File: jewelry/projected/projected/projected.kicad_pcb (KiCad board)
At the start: 2 copper layers, 28 x 28 mm, 38 parts, among them Q1 BC847, U1 STM32L432KBU6, U2 MCP73812T-420I-OT, U3 PCA9306DCUR, U4 MCP1640BCH, U5 TPS7A0533, U6 LIS2DE12

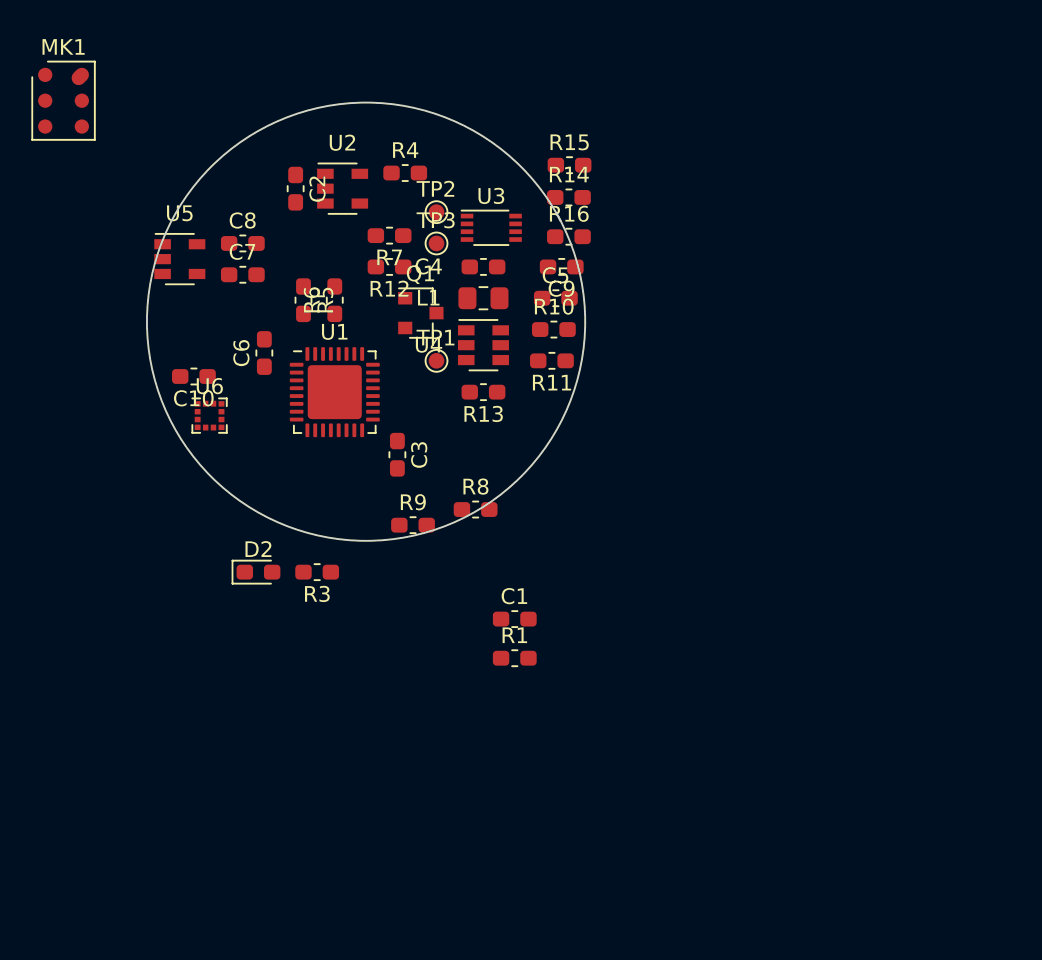
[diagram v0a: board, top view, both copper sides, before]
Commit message: projected: Layout nearly done
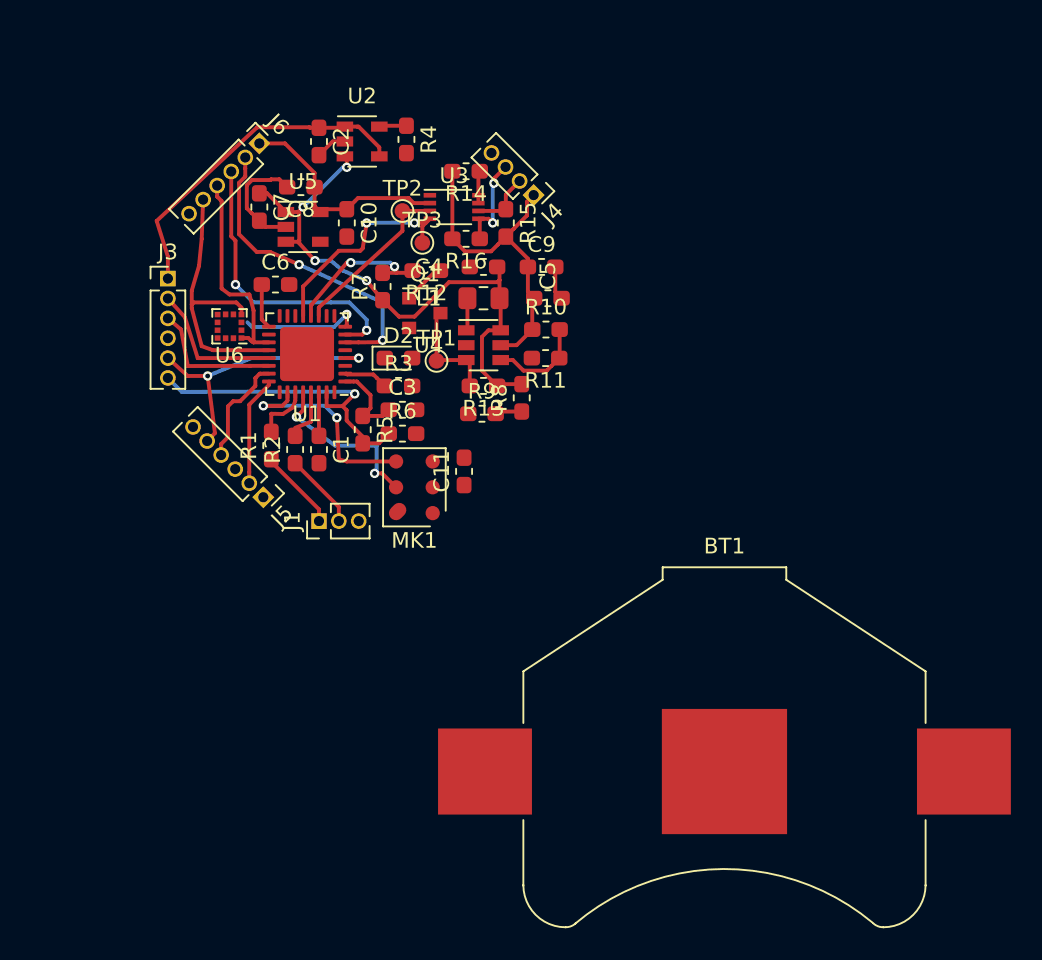
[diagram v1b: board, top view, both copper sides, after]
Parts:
- added BT1: LIR2450, Battery:BatteryHolder_Keystone_3008_1x2450, F.Cu at (72.9, 78.7)
- added C11: 1uF, Capacitor_SMD:C_0603_1608Metric_Pad1.05x0.95mm_HandSolder, F.Cu at (56.3, 59.6)
- added J1: TOUCH, Connector_PinHeader_1.27mm:PinHeader_1x03_P1.27mm_Vertical, F.Cu at (47.0, 62.7)
- added J3: DOCK, Connector_PinHeader_1.27mm:PinHeader_1x06_P1.27mm_Vertical, F.Cu at (37.3, 47.2)
- added J4: Leds, Connector_PinHeader_1.27mm:PinHeader_1x04_P1.27mm_Vertical, F.Cu at (60.7, 41.9)
- added J5: SWD, Connector_PinHeader_1.27mm:PinHeader_1x06_P1.27mm_Vertical, F.Cu at (43.4, 61.2)
- added J6: EXT, Connector_PinHeader_1.27mm:PinHeader_1x06_P1.27mm_Vertical, F.Cu at (43.2, 38.6)
- added R2: 1k, Resistor_SMD:R_0603_1608Metric_Pad1.05x0.95mm_HandSolder, F.Cu at (45.5, 58.2)
- R1: value R -> 1k
- moved MK1 33.4 mm to (53.1, 60.6), turned to 180 degrees
- moved R1 20.7 mm to (43.9, 57.9), turned to 90 degrees
- moved C1 16.5 mm to (47.0, 58.2), turned to 270 degrees
- moved D2 16.3 mm to (52.1, 52.3)
- moved C10 13.8 mm to (48.8, 43.7), turned to 270 degrees
- moved R3 13.0 mm to (52.1, 54.1), turned to 0 degrees
- moved R6 9.56 mm to (52.3, 57.1), turned to 0 degrees
- moved R5 9.10 mm to (49.8, 56.9)
- moved R9 8.37 mm to (57.4, 55.9)
- moved U5 8.14 mm to (46.0, 43.9)
- moved R8 7.72 mm to (59.9, 54.9), turned to 90 degrees
- moved R14 6.78 mm to (56.4, 40.4), turned to 180 degrees
- moved R16 6.57 mm to (56.4, 44.7), turned to 180 degrees
- moved U6 5.85 mm to (41.3, 50.3), turned to 180 degrees
- moved R15 5.49 mm to (58.9, 43.7), turned to 270 degrees
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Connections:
- C1 pad 1: Net-(C1-Pad1) -> /TOUCH_CS
- C1 pad 2: Net-(C1-Pad2) -> GND
- R1 pad 2: Net-(R1-Pad2) -> /TOUCH_1
- U1 pad 12: Net-(U1-Pad12) -> /LED_ENABLE
- U1 pad 18: /LED_ENABLE -> Net-(U1-Pad18)
- U1 pad 25: /TOUCH_2 -> Net-(U1-Pad25)
- U1 pad 27: Net-(U1-Pad27) -> /TOUCH_1
- U1 pad 29: Net-(U1-Pad29) -> /TOUCH_2
- U1 pad 30: /TOUCH_1 -> /TOUCH_CS
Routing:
- net +BATT: track 0.00 -> 37.4 mm, vias 0 -> 4
- net VCC: track 0.00 -> 22.7 mm
- net VBUS: track 0.00 -> 21.5 mm
- net +5V: track 0.00 -> 21.0 mm
- net /ANALOG+: track 0.00 -> 20.2 mm, vias 0 -> 2
- net /BOOT: track 0.00 -> 20.2 mm, vias 0 -> 1
- net /ANALOG-: track 0.00 -> 18.8 mm, vias 0 -> 2
- net /RESET: track 0.00 -> 18.1 mm, vias 0 -> 2
- net /I2C_SDA: track 0.00 -> 17.7 mm
- net /LED_DATA: track 0.00 -> 14.2 mm, vias 0 -> 2
- net /SAI_SCK: track 0.00 -> 13.6 mm, vias 0 -> 2
- net /I2C_SCL: track 0.00 -> 13.5 mm
- net /SAI_SD: track 0.00 -> 11.0 mm, vias 0 -> 2
- net /LED_CLK: track 0.00 -> 10.8 mm
- net /LED_ENABLE: track 0.00 -> 9.81 mm, vias 0 -> 2
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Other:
- board outline removed
- net class Default: via_dia 0.8 -> 0.6; via_drill 0.4 -> 0.3

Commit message: projected: Intial layout done
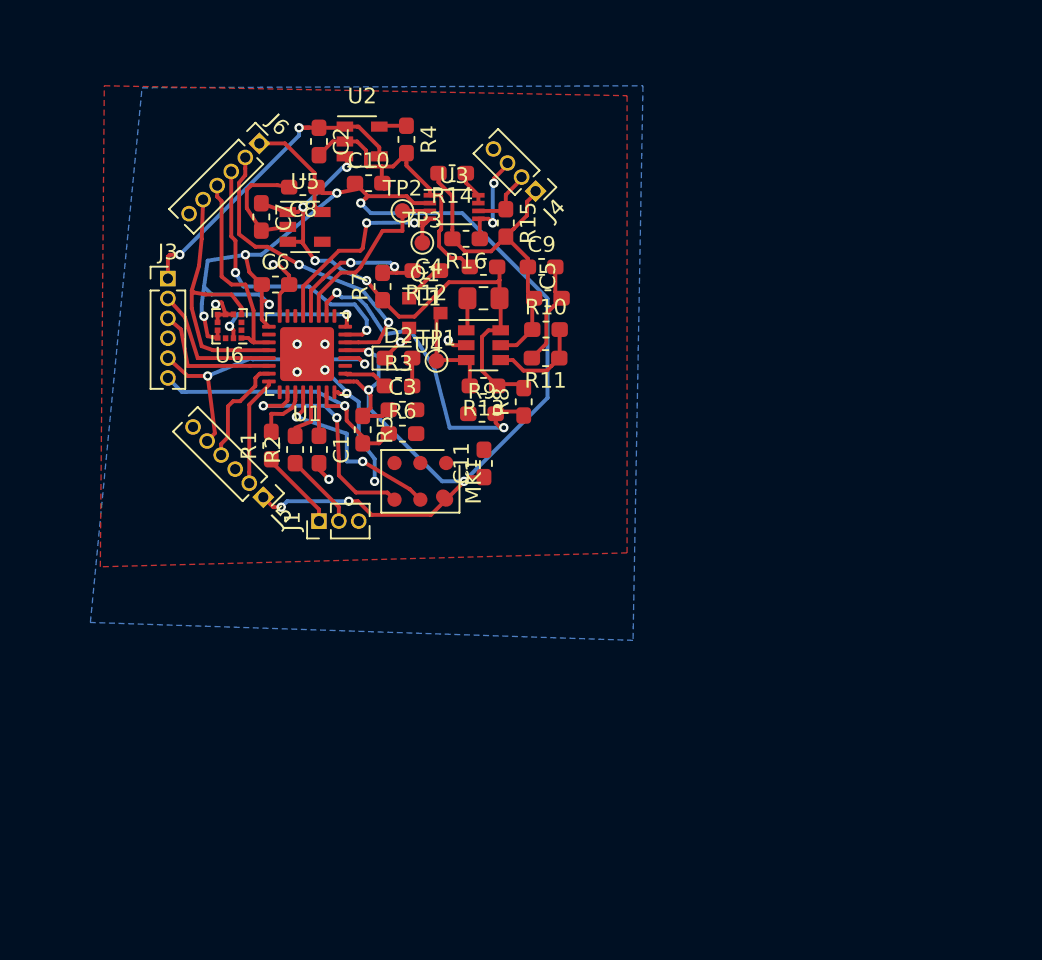
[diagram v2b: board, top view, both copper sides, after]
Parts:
- removed BT1: LIR2450, Battery:BatteryHolder_Keystone_3008_1x2450
- moved C10 2.90 mm to (50.2, 41.1), turned to 0 degrees
- moved C11 1.37 mm to (57.5, 59.1)
- moved R14 0.90 mm to (55.5, 40.5)
- moved C7 0.65 mm to (43.3, 43.3)
- moved MK1 0.54 mm to (53.5, 60.2), turned to 270 degrees
- moved R8 0.28 mm to (60.1, 55.1)
- moved J4 0.28 mm to (60.8, 41.7)
- moved C8 0.13 mm to (46.0, 41.4)
- moved U5 0.13 mm to (46.1, 43.9)
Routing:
- net VCC: track 22.7 -> 105.6 mm, vias 0 -> 10
- net GND: track 4.19 -> 47.3 mm, vias 0 -> 11
- net /BATT_SENSE: track 1.72 -> 21.0 mm, vias 0 -> 2
- net /ACCEL_INT: track 7.64 -> 9.60 mm, vias 1 -> 2
- net Net-(D2-Pad2): track 0.00 -> 1.78 mm
- net /SAI_SCK: track 13.6 -> 15.1 mm
- net /BOOT: track 20.2 -> 18.8 mm
- net /SAI_SD: track 11.0 -> 12.4 mm
- net VBUS: track 21.5 -> 20.4 mm, vias 0 -> 2
- net /RESET: track 18.1 -> 19.2 mm
- net /LED_CLK: track 10.8 -> 11.8 mm
- added copper zone on B.Cu, net GND
- added copper zone on F.Cu, net GND
